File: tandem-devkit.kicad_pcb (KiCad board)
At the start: 2 copper layers, 95.4 x 100 mm, 88 parts, among them J101 Conn_01x02, J102 QWIIC I2C Connector, J301 ConnectorLCDFrontLight, J302 FPC24(0.5MM), J303 FPC10(0.5MM), Q301 2N7002, Q302 2N7002, Q303 AO3401A, U201 AMS1117-ADJ_SOT223

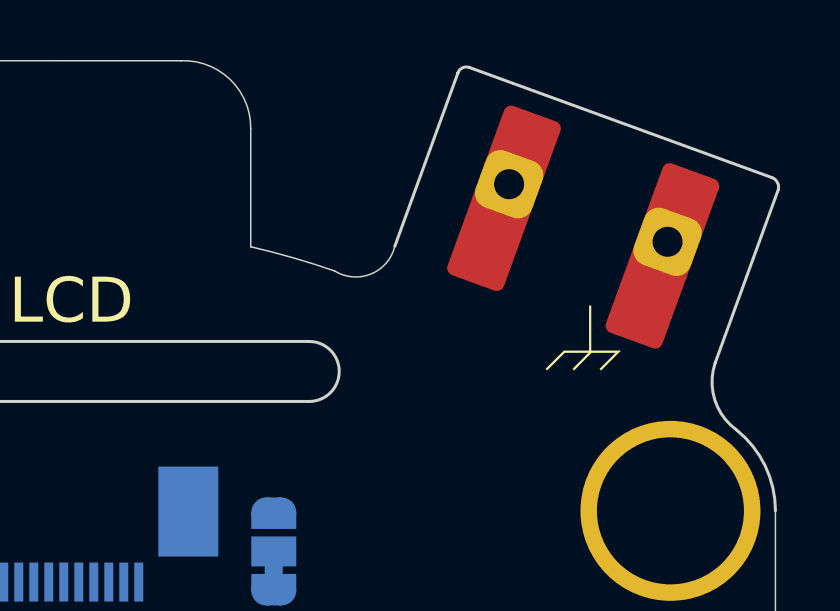
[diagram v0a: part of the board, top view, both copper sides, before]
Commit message: PCB: update netlist
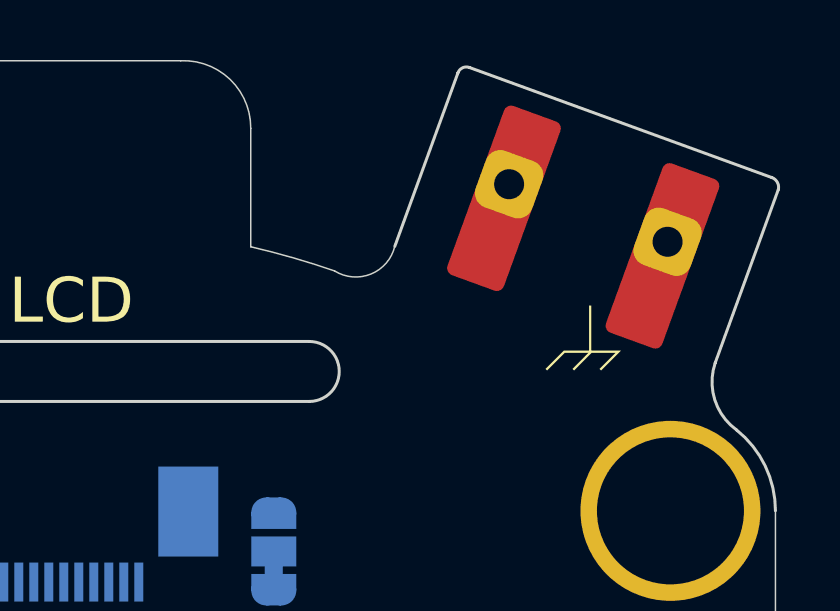
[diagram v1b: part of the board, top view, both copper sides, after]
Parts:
- renumbered R113 to R107, R107 to R108, R108 to R109, R112 to R110, R109 to R112, R110 to R113
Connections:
- A101 pad 10: Net-(A101-Pad10) -> /LCD_CURRENT_SENSE
- A101 pad 19: /CAP_TOUCH_2 -> Net-(A101-Pad19)
- A101 pad 20: Net-(A101-Pad20) -> unconnected-(A101-Pad20)
- A101 pad 25: /CAP_TOUCH_3 -> Net-(A101-Pad25)
- A101 pad 6: /EPD_CURRENT_SENSE -> /CAP_TOUCH_2
- A101 pad 7: /LCD_CURRENT_SENSE -> /CAP_TOUCH_3
- A101 pad 8: Net-(A101-Pad8) -> /CAP_TOUCH_4
- A101 pad 9: Net-(A101-Pad9) -> /EPD_CURRENT_SENSE
- A102 pad 10: Net-(A101-Pad10) -> /LCD_CURRENT_SENSE
- A102 pad 19: /CAP_TOUCH_2 -> Net-(A101-Pad19)
- A102 pad 20: Net-(A101-Pad20) -> unconnected-(A101-Pad20)
- A102 pad 25: /CAP_TOUCH_3 -> Net-(A101-Pad25)
- A102 pad 6: /EPD_CURRENT_SENSE -> /CAP_TOUCH_2
- A102 pad 7: /LCD_CURRENT_SENSE -> /CAP_TOUCH_3
- A102 pad 8: Net-(A101-Pad8) -> /CAP_TOUCH_4
- A102 pad 9: Net-(A101-Pad9) -> /EPD_CURRENT_SENSE
- R102 pad 2: Net-(A101-Pad20) -> Net-(A101-Pad19)
- R107 pad 2: Net-(A101-Pad10) -> Net-(A101-Pad25)
- R110 pad 2: Net-(A101-Pad9) -> Net-(A101-Pad15)
- R111 pad 2: Net-(A101-Pad8) -> Net-(A101-Pad16)
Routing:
- net Net-(A101-Pad9): track 6.13 -> 0.00 mm
- net Net-(A101-Pad10): track 6.13 -> 0.00 mm
- net Net-(A101-Pad25): track 0.00 -> 6.13 mm
- net Net-(A101-Pad19): track 0.00 -> 6.13 mm
- net Net-(A101-Pad8): track 6.13 -> 0.00 mm
- net /CAP_TOUCH_4: track 0.00 -> 6.13 mm
